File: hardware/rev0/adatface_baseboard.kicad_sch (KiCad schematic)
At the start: 89 parts, among them J1 Conn_01x06_Male, J2 Conn_02x32_Odd_Even, J3 Conn_02x32_Odd_Even, J4 Connector_USB_C_Receptacle_US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, J5 Connector_USB_C_Receptacle_US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, J6 Conn_01x06_Male, J7 Conn_01x23_Male, J8 Conn_01x01_Male, J9 Conn_01x01_Male, U1 PLR135-T10, U2 PLR135-T10, U3 PLR135-T10, U4 PLR135-T10, U5 USB3320, U6 USB3320, U7 ME6212C18M5G

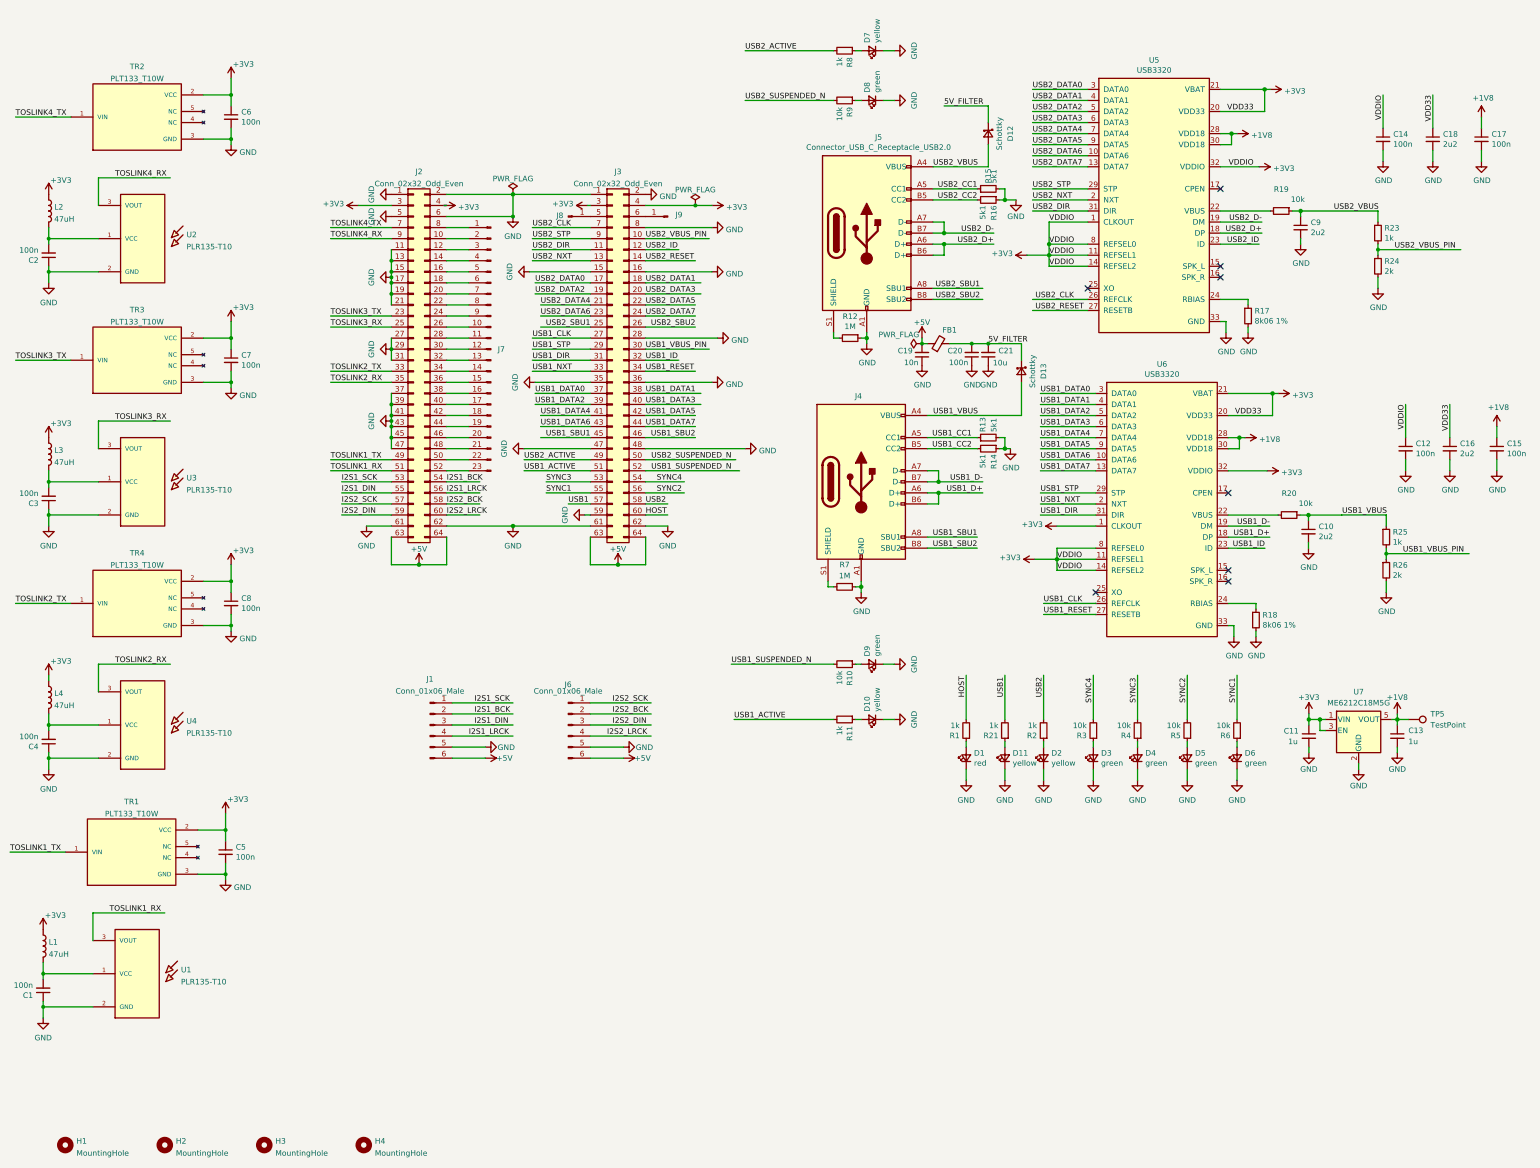
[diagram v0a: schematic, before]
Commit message: Fix bugs in rev0
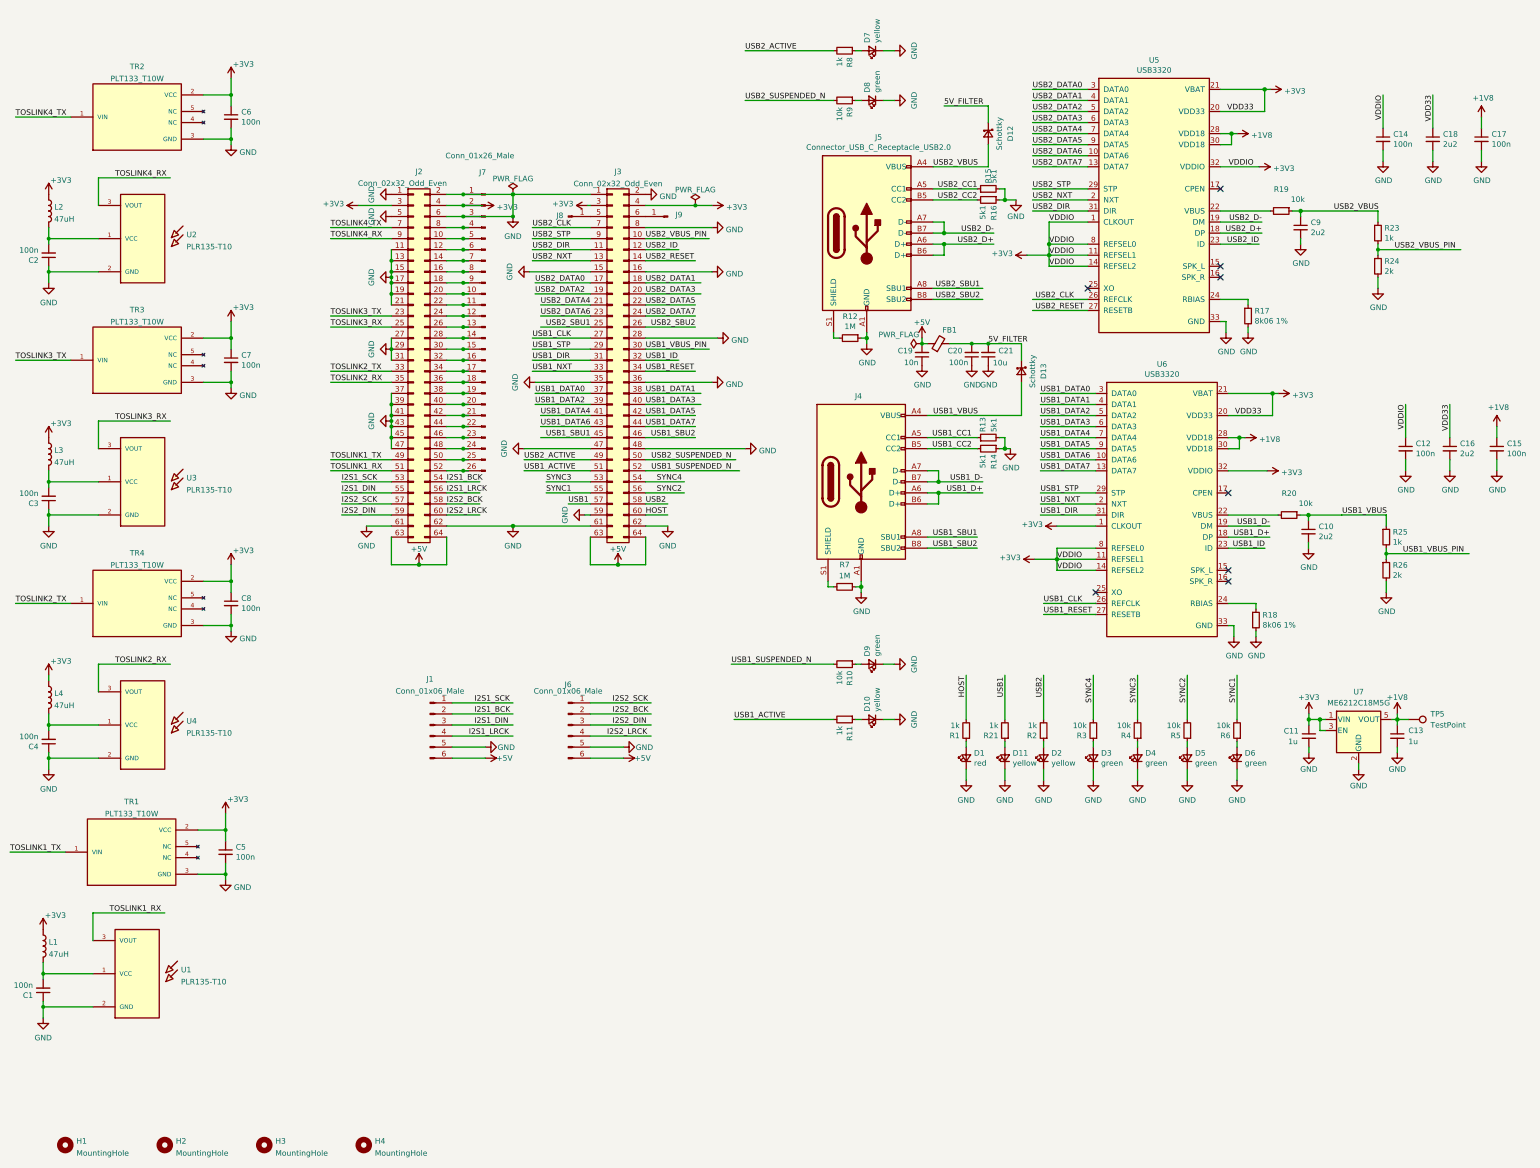
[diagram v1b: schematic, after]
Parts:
- removed J7: Conn_01x23_Male, Connector_PinHeader_2.54mm:PinHeader_1x23_P2.54mm_Vertical, symbol Connector:Conn_01x23_Male
- added J7: Conn_01x26_Male, Connector_PinHeader_2.54mm:PinHeader_1x26_P2.54mm_Horizontal, symbol Connector:Conn_01x26_Male
- J8, J9: footprint Connector_PinHeader_2.54mm:PinHeader_1x01_P2.54mm_Vertical -> Connector_PinHeader_2.54mm:PinHeader_1x01_P2.54mm_Horizontal
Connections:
- net +3V3: now also J7.2 (Pin_2)
- net GND: now also J7.1 (Pin_1), J7.3 (Pin_3)
- net at J2.8 (Pin_8): now also J7.4 (Pin_4)
- net at J2.26 (Pin_26): now also J7.13 (Pin_13)
- net at J2.28 (Pin_28): now also J7.14 (Pin_14)
- net at J2.30 (Pin_30): now also J7.15 (Pin_15)
- net at J2.32 (Pin_32): now also J7.16 (Pin_16)
- net at J2.34 (Pin_34): now also J7.17 (Pin_17)
- net at J2.36 (Pin_36): now also J7.18 (Pin_18)
- net at J2.38 (Pin_38): now also J7.19 (Pin_19)
- net at J2.40 (Pin_40): now also J7.20 (Pin_20)
- net at J2.42 (Pin_42): now also J7.21 (Pin_21)
- net at J2.44 (Pin_44): now also J7.22 (Pin_22)
- net at J2.10 (Pin_10): now also J7.5 (Pin_5)
- net at J2.46 (Pin_46): now also J7.23 (Pin_23)
- net at J2.48 (Pin_48): now also J7.24 (Pin_24)
- net at J2.50 (Pin_50): now also J7.25 (Pin_25)
- net at J2.52 (Pin_52): now also J7.26 (Pin_26)
- net at J2.12 (Pin_12): now also J7.6 (Pin_6)
- net at J2.14 (Pin_14): now also J7.7 (Pin_7)
- net at J2.16 (Pin_16): now also J7.8 (Pin_8)
- net at J2.18 (Pin_18): now also J7.9 (Pin_9)
- net at J2.20 (Pin_20): now also J7.10 (Pin_10)
- net at J2.22 (Pin_22): now also J7.11 (Pin_11)
- net at J2.24 (Pin_24): now also J7.12 (Pin_12)
